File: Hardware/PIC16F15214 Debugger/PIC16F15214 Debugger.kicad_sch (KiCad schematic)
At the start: 4 parts, among them J1 2-Pin Terminal, J2 5-Pin-Header, Q1 AOI21357, U1 PIC16F15214

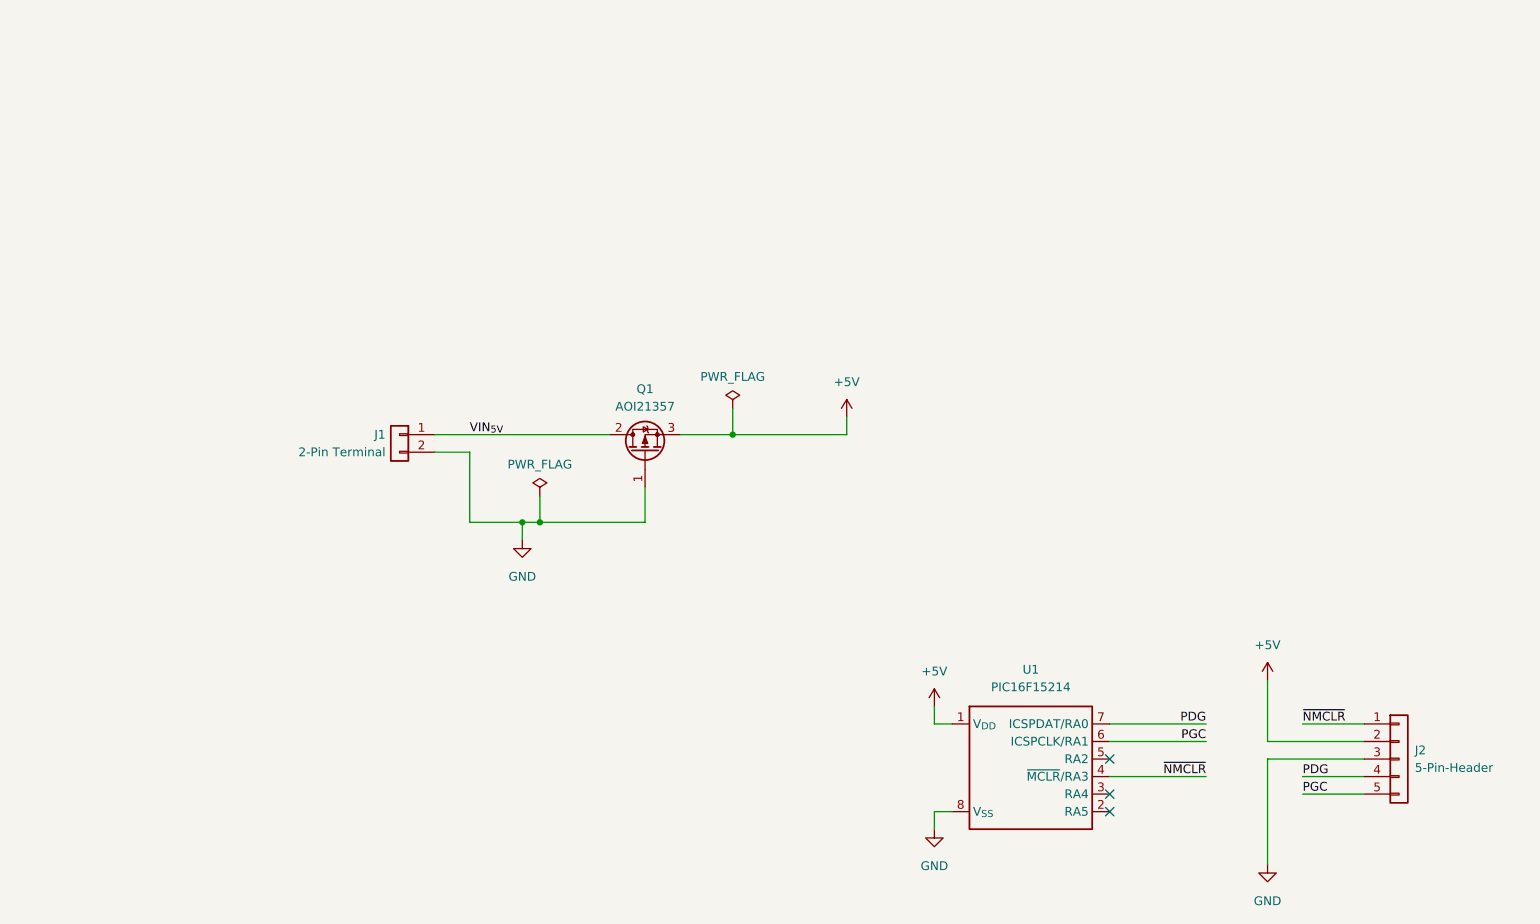
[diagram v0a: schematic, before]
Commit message: Final Version, project finished
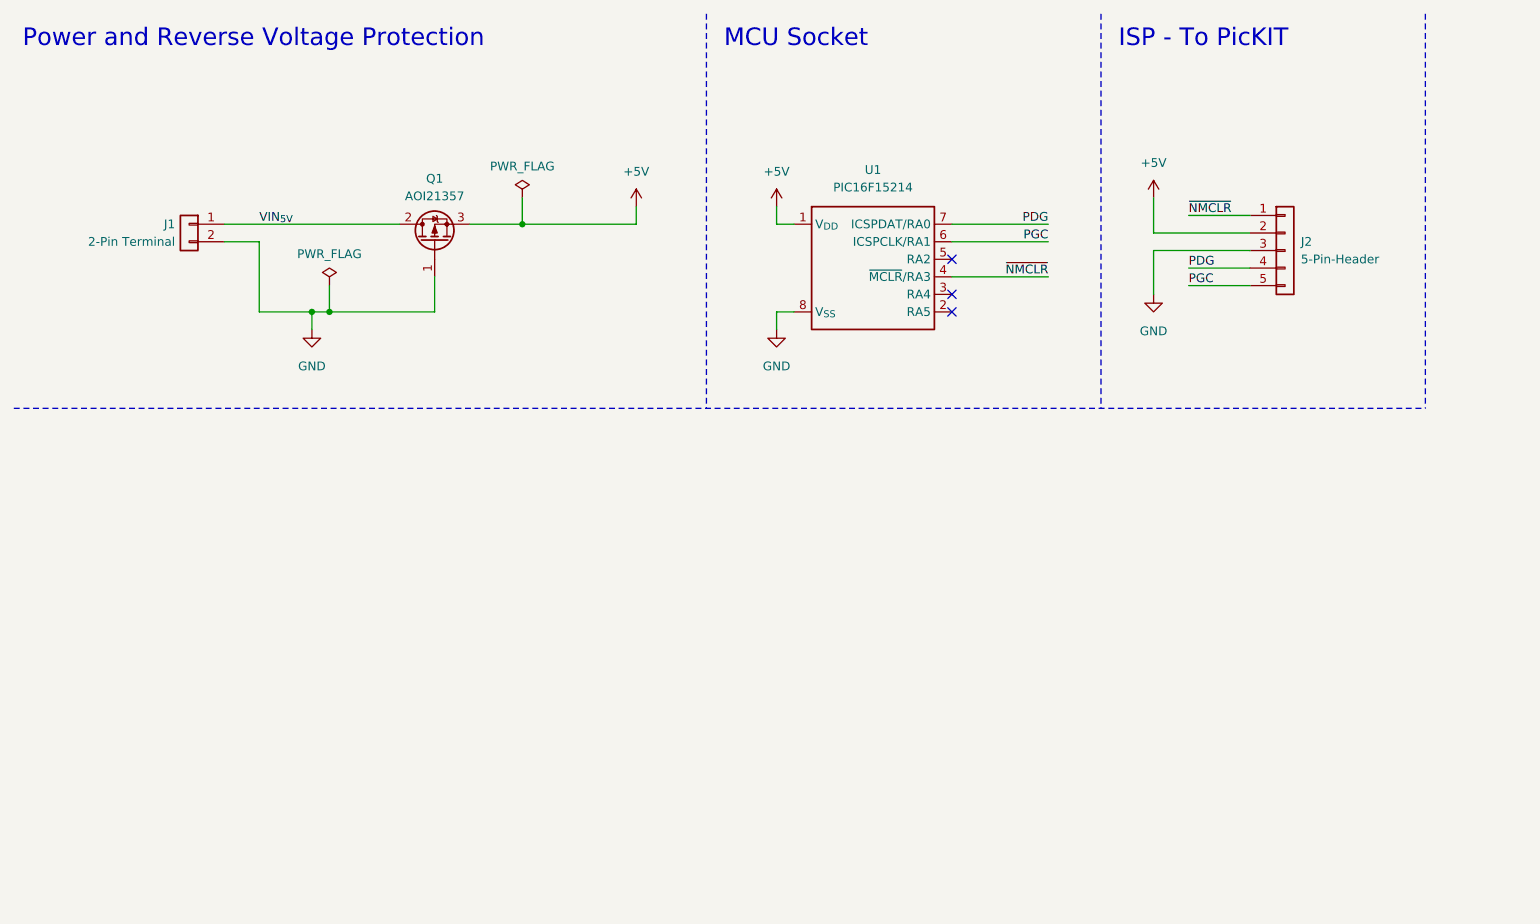
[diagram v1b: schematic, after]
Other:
- note added: "ISP - To PicKIT"
- note added: "MCU Socket"
- note added: "Power and Reverse Voltage Protection"
- moved on the sheet: J1, J2, Q1, U1
